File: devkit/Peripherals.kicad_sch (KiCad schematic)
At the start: 50 parts, among them IC501 APDS-9306-065, IC502 BMI270, IC503 LIS2MDLTR, IC504 BMP581, IC505 DRV2603RUNT, IC506 PCA9306JK, IC507 RV-8263-C8, J501 Jumper, J502 Jumper, J503 Jumper, J504 Jumper, J505 Jumper, J506 Jumper, J507 Jumper, M501 Vibrator DC Motor, X501 Current, X502 I2S, X503 Current, X504 I2C, X505 Current, X506 Current, X507 Current, X508 Current, X509 Motor, X510 Current

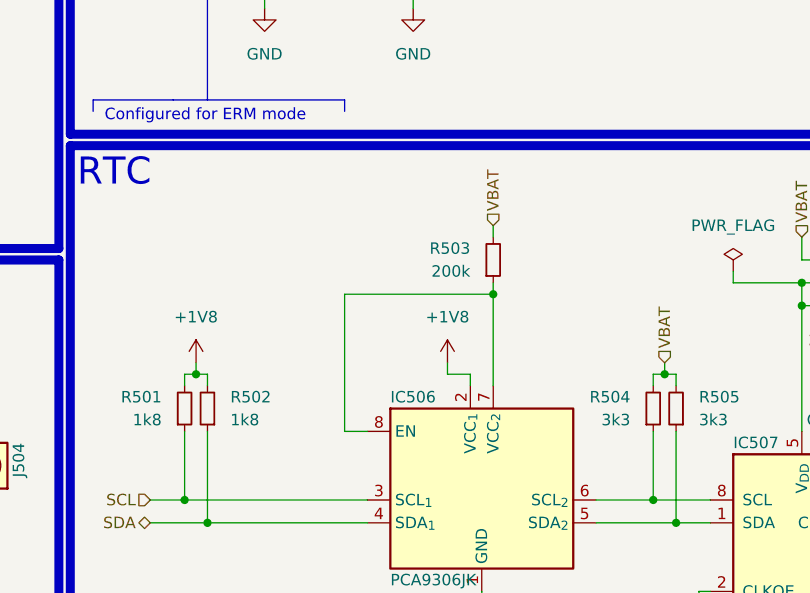
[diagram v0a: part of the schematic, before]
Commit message: Revert "Bug: Issue #172"
This reverts commit d2b21792fba04b32ee89f1631bab4de80096e44a.
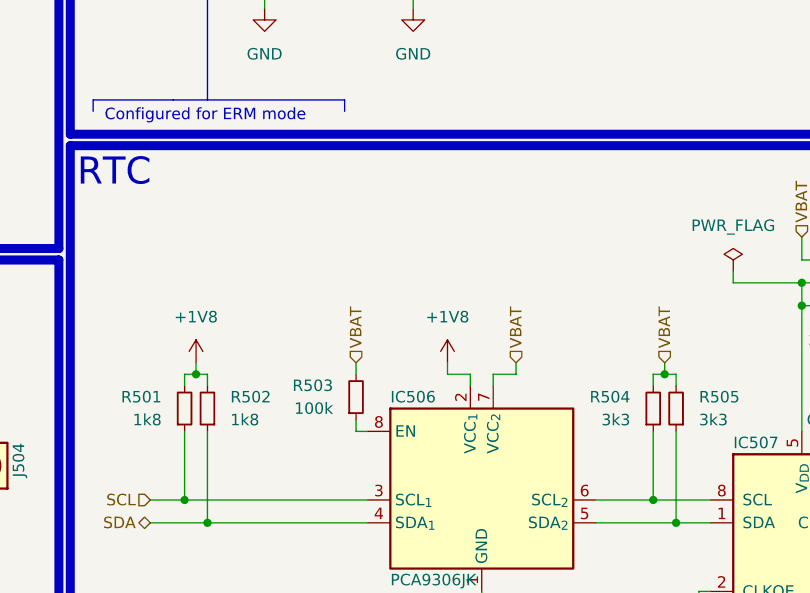
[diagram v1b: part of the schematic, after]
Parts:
- R503: value 200k -> 100k; manf# RC0402FR-07200KL -> RC0402FR-07100KL; mouser# 603-RC0402FR-07200KL -> 603-RC0402FR-07100KL
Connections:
- net VBAT: now also IC506.7 (VCC_{2})
- net at IC506.8 (EN), R503.1: no longer IC506.7 (VCC_{2})
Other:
- moved on the sheet: R503
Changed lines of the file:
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@@
 	)
 	(junction
-		(at 346.71 109.22)
-		(diameter 0)
-		(color 0 0 0 0)
-	)
-	(junction
 		(at 19.05 111.76)
 		(diameter 0)
@@
 	(wire
 		(pts
-			(xy 346.71 107.95) (xy 346.71 109.22)
+			(xy 331.47 123.19) (xy 331.47 124.46)
 		)
 		(stroke
@@
 	(wire
 		(pts
-			(xy 346.71 101.6) (xy 346.71 102.87)
+			(xy 331.47 116.84) (xy 331.47 118.11)
 		)
 		(stroke
@@
 	(wire
 		(pts
+			(xy 349.25 116.84) (xy 349.25 118.11)
+		)
+		(stroke
+			(width 0)
+			(type default)
+		)
+	)
+	(wire
+		(pts
 			(xy 199.39 43.18) (xy 199.39 45.72)
 		)
@@
 	(wire
 		(pts
-			(xy 330.2 109.22) (xy 346.71 109.22)
-		)
-		(stroke
-			(width 0)
-			(type default)
-		)
-	)
-	(wire
-		(pts
 			(xy 196.85 93.98) (xy 196.85 95.25)
 		)
@@
 	(wire
 		(pts
-			(xy 330.2 124.46) (xy 332.74 124.46)
+			(xy 331.47 124.46) (xy 332.74 124.46)
 		)
 		(stroke
@@
 	(wire
 		(pts
-			(xy 346.71 109.22) (xy 346.71 119.38)
+			(xy 346.71 118.11) (xy 346.71 119.38)
 		)
 		(stroke
@@
 	(wire
 		(pts
-			(xy 330.2 109.22) (xy 330.2 124.46)
-		)
-		(stroke
-			(width 0)
-			(type default)
-		)
-	)
-	(wire
-		(pts
 			(xy 313.69 118.11) (xy 313.69 116.84)
 		)
@@
 	(wire
 		(pts
+			(xy 349.25 118.11) (xy 346.71 118.11)
+		)
+		(stroke
+			(width 0)
+			(type default)
+		)
+	)
+	(wire
+		(pts
 			(xy 364.49 132.08) (xy 370.84 132.08)
 		)
@@
 		)
 	)
+	(hierarchical_label "VBAT"
+		(shape input)
+		(at 349.25 116.84 90)
+		(effects
+			(font
+				(size 1.27 1.27)
+			)
+			(justify left)
+		)
+	)
 	(hierarchical_label "SDA"
 		(shape bidirectional)
@@
 	(hierarchical_label "VBAT"
 		(shape input)
-		(at 346.71 101.6 90)
+		(at 331.47 116.84 90)
 		(effects
 			(font
@@
 	(symbol
 		(lib_id "Device:R_Small")
-		(at 346.71 105.41 0)
+		(at 331.47 120.65 0)
 		(mirror x)
 		(unit 1)
@@
 		(fields_autoplaced yes)
 		(property "Reference" "R503"
-			(at 344.17 104.14 0)
+			(at 328.93 119.38 0)
 			(effects
 				(font
@@
 			)
 		)
-		(property "Value" "200k"
-			(at 344.17 106.68 0)
+		(property "Value" "100k"
+			(at 328.93 121.92 0)
 			(effects
 				(font
@@
 		)
 		(property "Footprint" "Resistor_SMD:R_0402_1005Metric"
-			(at 346.71 105.41 0)
+			(at 331.47 120.65 0)
 			(effects
 				(font
@@
 		)
 		(property "Datasheet" "https://www.mouser.com/catalog/specsheets/YAGEO_PYu_RC_Group_51_RoHS_L_12.pdf"
-			(at 346.71 105.41 0)
+			(at 331.47 120.65 0)
 			(effects
 				(font
@@
 		)
 		(property "Description" "Resistor, small symbol"
-			(at 346.71 105.41 0)
+			(at 331.47 120.65 0)
 			(effects
 				(font
@@
 		)
 		(property "CONFIG" ""
-			(at 346.71 105.41 0)
+			(at 331.47 120.65 0)
 			(effects
 				(font
@@
 		)
 		(property "manf" "YAGEO"
-			(at 346.71 105.41 0)
+			(at 331.47 120.65 0)
 			(effects
 				(font
@@
 			)
 		)
-		(property "manf#" "RC0402FR-07200KL"
-			(at 346.71 105.41 0)
+		(property "manf#" "RC0402FR-07100KL"
+			(at 331.47 120.65 0)
 			(effects
 				(font
@@
 			)
 		)
-		(property "mouser#" "603-RC0402FR-07200KL"
-			(at 346.71 105.41 0)
+		(property "mouser#" "603-RC0402FR-07100KL"
+			(at 331.47 120.65 0)
 			(effects
 				(font
